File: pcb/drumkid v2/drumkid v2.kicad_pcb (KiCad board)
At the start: 2 copper layers, 0 parts

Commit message: more pcb changes, about to do a big-ish change so doing a commit now
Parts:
- added BT1: Battery, Connector_PinHeader_2.54mm:PinHeader_1x02_P2.54mm_Vertical, F.Cu at (162.0, 128.0)
- added C1: 150uF, Capacitor_THT:CP_Radial_D6.3mm_P2.50mm, F.Cu at (137.0, 64.0)
- added C10: 220uF, Capacitor_THT:CP_Radial_D6.3mm_P2.50mm, F.Cu at (102.0, 71.0)
- added C2: 0.1uF, Capacitor_THT:C_Disc_D3.4mm_W2.1mm_P2.50mm, F.Cu at (150.0, 55.0)
- added C3: 100uF, Capacitor_THT:CP_Radial_D6.3mm_P2.50mm, F.Cu at (137.0, 56.0)
- added C4: 0.1uF, Capacitor_THT:C_Disc_D3.4mm_W2.1mm_P2.50mm, F.Cu at (113.0, 53.0)
- added C5: 10uF, Capacitor_THT:C_Disc_D3.4mm_W2.1mm_P2.50mm, F.Cu at (142.0, 84.0)
- added C6: 10uF, Capacitor_THT:C_Disc_D3.4mm_W2.1mm_P2.50mm, F.Cu at (147.0, 84.0)
- added C7: 10uF, Capacitor_THT:CP_Radial_D6.3mm_P2.50mm, F.Cu at (114.0, 60.0)
- added C8: 100uF, Capacitor_THT:CP_Radial_D6.3mm_P2.50mm, F.Cu at (94.0, 71.0)
- added C9: 0.1uF, Capacitor_THT:C_Disc_D3.4mm_W2.1mm_P2.50mm, F.Cu at (92.0, 79.0)
- added D1: 1N5817, Diode_THT:D_DO-41_SOD81_P10.16mm_Horizontal, F.Cu at (144.0, 65.0)
- added D2: LED, LED_THT:LED_D5.0mm, F.Cu at (151.0, 72.0)
- added D3: LED, LED_THT:LED_D5.0mm, F.Cu at (111.0, 72.0)
- added D4: LED, LED_THT:LED_D5.0mm, F.Cu at (121.0, 72.0)
- added D5: LED, LED_THT:LED_D5.0mm, F.Cu at (131.0, 72.0)
- added D6: LED, LED_THT:LED_D5.0mm, F.Cu at (141.0, 72.0)
- added J1: Conn_01x03_Female, Connector_PinHeader_2.54mm:PinHeader_1x03_P2.54mm_Vertical, F.Cu at (169.0, 67.7)
- added J2: Conn_01x03_Female, Connector_PinHeader_2.54mm:PinHeader_1x03_P2.54mm_Vertical, F.Cu at (154.0, 63.0)
- added J3: Conn_01x03_Female, Connector_PinHeader_2.54mm:PinHeader_1x03_P2.54mm_Vertical, F.Cu at (169.0, 64.0)
- added J4: Conn_01x03_Female, Connector_PinHeader_2.54mm:PinHeader_1x03_P2.54mm_Vertical, F.Cu at (154.1, 66.0)
- added J5: Conn_01x05_Female, Connector_PinHeader_2.54mm:PinHeader_1x05_P2.54mm_Vertical, F.Cu at (122.0, 54.0)
- added J6: Conn_01x04_Female, Connector_PinHeader_2.54mm:PinHeader_1x04_P2.54mm_Vertical, F.Cu at (153.0, 77.0)
- added J7: Conn_01x06_Female, Connector_PinHeader_2.54mm:PinHeader_1x06_P2.54mm_Vertical, F.Cu at (169.0, 61.0)
- added J8: Conn_01x05_Female, Connector_PinHeader_2.54mm:PinHeader_1x05_P2.54mm_Vertical, F.Cu at (169.0, 81.0)
- added J9: AudioJack3_Ground_Switch, headphone:Tayda_3.5mm_stereo_TRS_jack_A-853, F.Cu at (105.0, 38.0)
- added L1: L, Inductor_THT:L_Radial_D6.0mm_P4.00mm, F.Cu at (128.0, 64.0)
- added R1: 470, Resistor_THT:R_Axial_DIN0207_L6.3mm_D2.5mm_P10.16mm_Horizontal, F.Cu at (123.0, 46.0)
- added R10: 100k, Resistor_THT:R_Axial_DIN0207_L6.3mm_D2.5mm_P10.16mm_Horizontal, F.Cu at (97.0, 64.0)
- added R2: 10k, Resistor_THT:R_Axial_DIN0207_L6.3mm_D2.5mm_P10.16mm_Horizontal, F.Cu at (155.0, 45.0)
- added R3: 220, Resistor_THT:R_Axial_DIN0207_L6.3mm_D2.5mm_P10.16mm_Horizontal, F.Cu at (113.0, 87.0)
- added R4: 220, Resistor_THT:R_Axial_DIN0207_L6.3mm_D2.5mm_P10.16mm_Horizontal, F.Cu at (117.0, 87.0)
- added R5: 220, Resistor_THT:R_Axial_DIN0207_L6.3mm_D2.5mm_P10.16mm_Horizontal, F.Cu at (121.0, 87.0)
- added R6: 220, Resistor_THT:R_Axial_DIN0207_L6.3mm_D2.5mm_P10.16mm_Horizontal, F.Cu at (125.0, 87.0)
- added R7: 220, Resistor_THT:R_Axial_DIN0207_L6.3mm_D2.5mm_P10.16mm_Horizontal, F.Cu at (129.0, 77.0)
- added R8: 10, Resistor_THT:R_Axial_DIN0207_L6.3mm_D2.5mm_P10.16mm_Horizontal, F.Cu at (108.0, 79.0)
- added R9: 470k, Resistor_THT:R_Axial_DIN0207_L6.3mm_D2.5mm_P10.16mm_Horizontal, F.Cu at (93.0, 64.0)
- added REF**: MountingHole_3.2mm_M3, MountingHole:MountingHole_3.2mm_M3, F.Cu at (94.0, 39.0)
- added REF**: MountingHole_3.2mm_M3, MountingHole:MountingHole_3.2mm_M3, F.Cu at (171.0, 126.0)
- added REF**: MountingHole_3.2mm_M3, MountingHole:MountingHole_3.2mm_M3, F.Cu at (171.0, 39.0)
- added REF**: MountingHole_3.2mm_M3, MountingHole:MountingHole_3.2mm_M3, F.Cu at (94.0, 126.0)
- added RV1: R_POT, SamacSys_Parts:RK14J12A0A0K, F.Cu at (132.0, 46.0)
- added RV2: R_POT, Potentiometer_THT:Potentiometer_Bourns_PTV09A-1_Single_Vertical, F.Cu at (110.0, 90.0)
- added RV3: R_POT, Potentiometer_THT:Potentiometer_Bourns_PTV09A-1_Single_Vertical, F.Cu at (150.0, 90.0)
- added RV4: R_POT, Potentiometer_THT:Potentiometer_Bourns_PTV09A-1_Single_Vertical, F.Cu at (130.0, 90.0)
- added SW1: SW_SPDT, SamacSys_Parts:EG1206, F.Cu at (160.0, 37.0)
- added SW2: SW_Push, Button_Switch_THT:SW_PUSH-12mm_Wuerth-430476085716, F.Cu at (94.0, 119.0)
- added SW3: SW_Push, Button_Switch_THT:SW_PUSH-12mm_Wuerth-430476085716, F.Cu at (108.0, 119.0)
- added SW4: SW_Push, Button_Switch_THT:SW_PUSH-12mm_Wuerth-430476085716, F.Cu at (140.0, 123.0)
- added SW5: SW_Push, Button_Switch_THT:SW_PUSH-12mm_Wuerth-430476085716, F.Cu at (153.0, 120.0)
- added SW6: SW_Push, Button_Switch_THT:SW_PUSH-12mm_Wuerth-430476085716, F.Cu at (166.0, 117.0)
- added U1: MAX756, Package_DIP:DIP-8_W7.62mm_Socket, F.Cu at (144.0, 51.0)
- added U2: ATmega328P-PU, Package_DIP:DIP-28_W7.62mm_Socket, F.Cu at (158.0, 48.0)
- added U3: LM386, Package_DIP:DIP-8_W7.62mm_Socket, F.Cu at (101.0, 56.0)
- added Y1: Crystal, Crystal:Crystal_HC49-4H_Vertical, F.Cu at (142.0, 80.0)
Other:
- board outline added: 85 x 95 mm

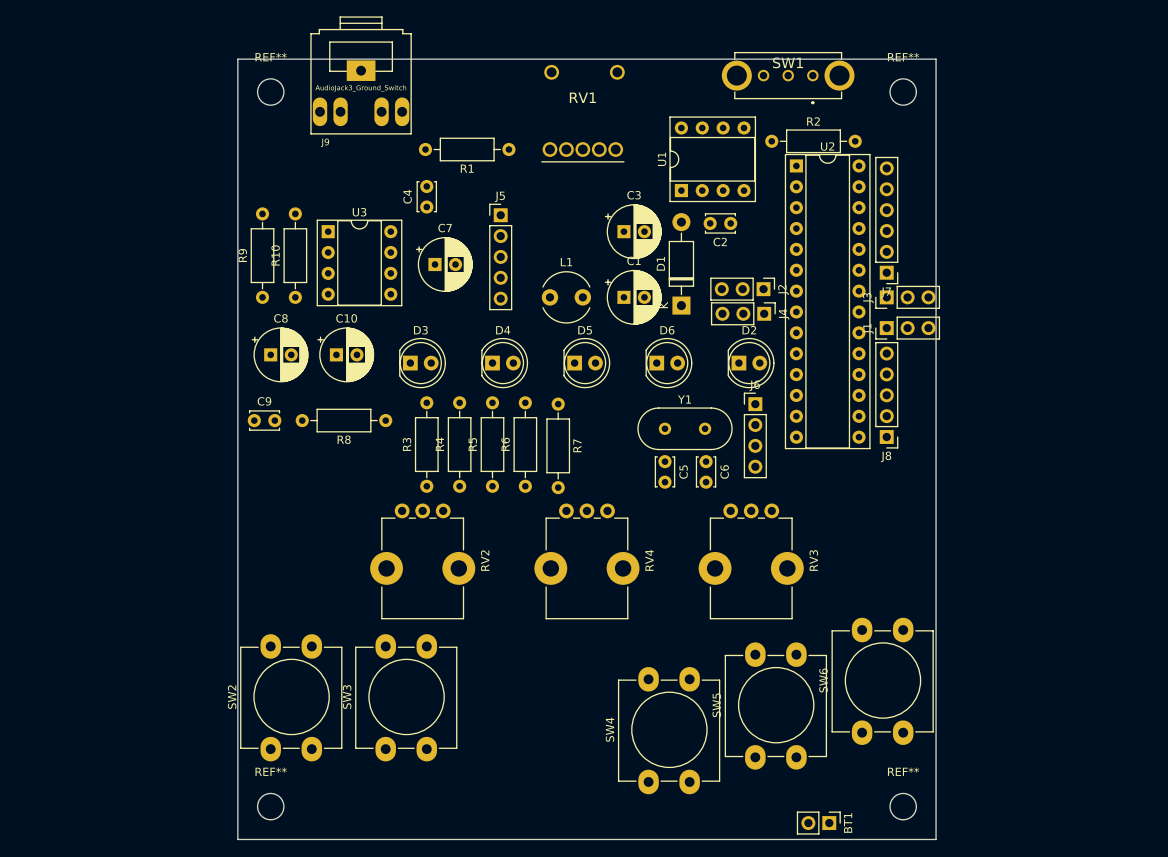
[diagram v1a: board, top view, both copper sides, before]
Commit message: good pcb progress, about to make a little change
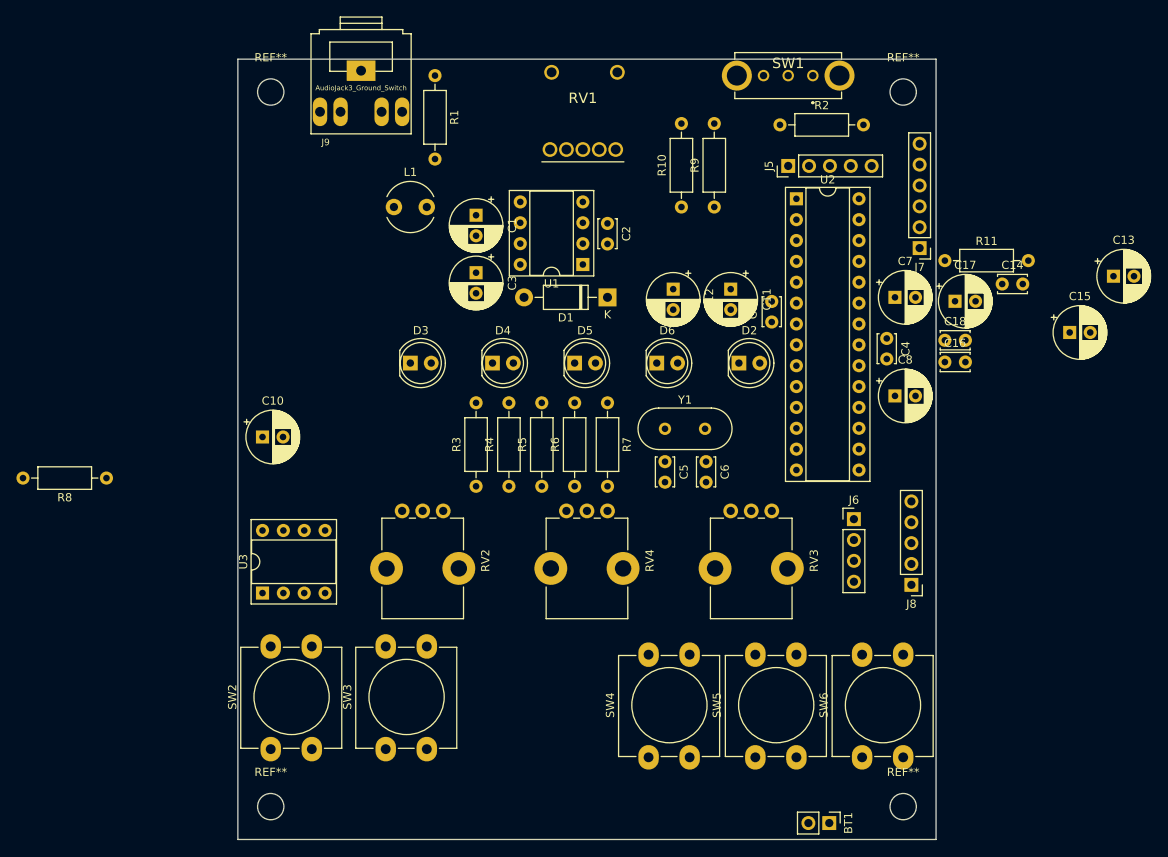
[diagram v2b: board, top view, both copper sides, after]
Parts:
- removed J1, J2, J3, J4: Conn_01x03_Female, Connector_PinHeader_2.54mm:PinHeader_1x03_P2.54mm_Vertical
- added C11: CP, Capacitor_THT:CP_Radial_D6.3mm_P2.50mm, F.Cu at (150.0, 63.0)
- added C12: CP, Capacitor_THT:CP_Radial_D6.3mm_P2.50mm, F.Cu at (143.0, 63.0)
- added C13: 2.2uF, Capacitor_THT:CP_Radial_D6.3mm_P2.50mm, F.Cu at (196.6, 61.4)
- added C14: 220nF, Capacitor_THT:C_Disc_D3.4mm_W2.1mm_P2.50mm, F.Cu at (183.1, 62.4)
- added C15: 10uF, Capacitor_THT:CP_Radial_D6.3mm_P2.50mm, F.Cu at (191.3, 68.3)
- added C16: 100nF, Capacitor_THT:C_Disc_D3.4mm_W2.1mm_P2.50mm, F.Cu at (176.1, 71.9)
- added C17: 10uF, Capacitor_THT:CP_Radial_D6.3mm_P2.50mm, F.Cu at (177.3, 64.5)
- added C18: 100nF, Capacitor_THT:C_Disc_D3.4mm_W2.1mm_P2.50mm, F.Cu at (176.1, 69.2)
- added R11: 10, Resistor_THT:R_Axial_DIN0207_L6.3mm_D2.5mm_P10.16mm_Horizontal, F.Cu at (176.1, 59.5)
- C4, C9: value 0.1uF -> C
- C7: value 10uF -> CP
- C8: value 100uF -> CP
- R1: value 470 -> 47
- R10: value 100k -> 1k
- R8: value 10 -> 470
- R9: value 470k -> 10k
- RV1: value R_POT -> 10k
- moved C8 76.2 mm to (170.0, 76.0)
- moved C9 64.1 mm to (155.0, 67.0), turned to 90 degrees
- moved C4 58.2 mm to (169.0, 69.0), turned to 270 degrees
- moved C7 56.1 mm to (170.0, 64.0)
- moved R9 56.1 mm to (148.0, 53.0)
- moved R10 48.3 mm to (144.0, 53.0)
- moved U3 44.7 mm to (93.0, 100.0), turned to 90 degrees
- moved J5 35.5 mm to (157.0, 48.0), turned to 90 degrees
- moved R8 34.7 mm to (74.0, 86.0)
- moved L1 22.0 mm to (109.0, 53.0)
- moved C1 20.6 mm to (119.0, 54.0), turned to 270 degrees
- moved C3 18.7 mm to (119.0, 61.0), turned to 270 degrees
- moved J6 18.4 mm to (165.0, 91.0)
- moved J8 18.2 mm to (172.0, 99.0)
- moved C2 15.0 mm to (135.0, 55.0), turned to 270 degrees
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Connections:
- C4 pad 2: Net-(C4-Pad2) -> +5V
- C7 pad 1: Net-(C7-Pad1) -> +5V
- C9 pad 1: Net-(C10-Pad1) -> GND
- C9 pad 2: Net-(C9-Pad2) -> +5V
- R1 pad 1: /DIGITAL_9 -> Net-(C13-Pad1)
- R1 pad 2: Net-(C4-Pad2) -> /DIGITAL_9
- R10 pad 1: GND -> Net-(R10-Pad1)
- R10 pad 2: Net-(R10-Pad2) -> GND
- R8 pad 1: GND -> Net-(C14-Pad1)
- R8 pad 2: Net-(C9-Pad2) -> Net-(C13-Pad1)
- R9 pad 1: Net-(C4-Pad2) -> Net-(R10-Pad1)
- R9 pad 2: Net-(R10-Pad2) -> Net-(C15-Pad2)
- RV1 pad 1: GND -> Net-(RV1-Pad1)
- RV1 pad 3: Net-(R10-Pad2) -> Net-(R10-Pad1)
- U3 pad 2: GND -> Net-(RV1-Pad1)
- U3 pad 4: GND -> Net-(C16-Pad2)
- U3 pad 7: Net-(C7-Pad1) -> Net-(C17-Pad2)
